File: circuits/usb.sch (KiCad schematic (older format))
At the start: 18 parts, among them J18 USB_MINI_B, Q5 Crystal_12Mhz, Q6 Q_SS8050, Q7 Q_SS8550, U10 CH340T(SSOP20W)

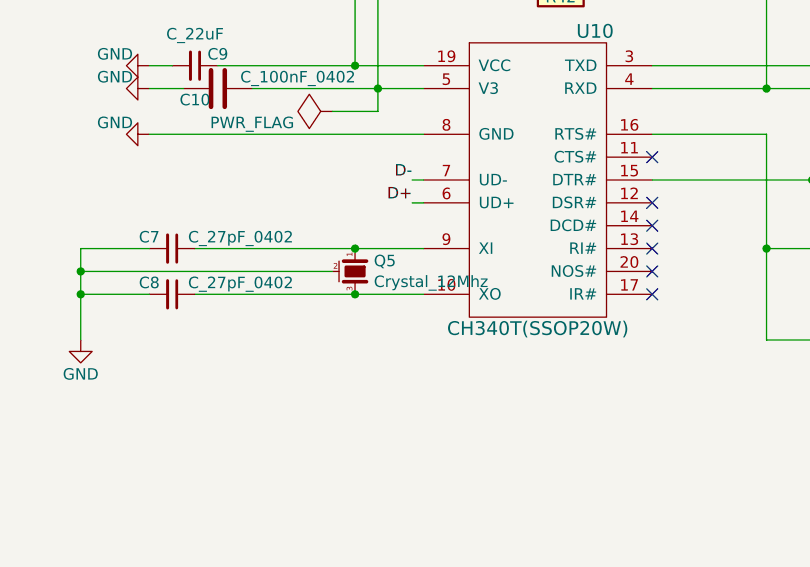
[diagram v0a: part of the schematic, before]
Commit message: finished layout, sent to board house
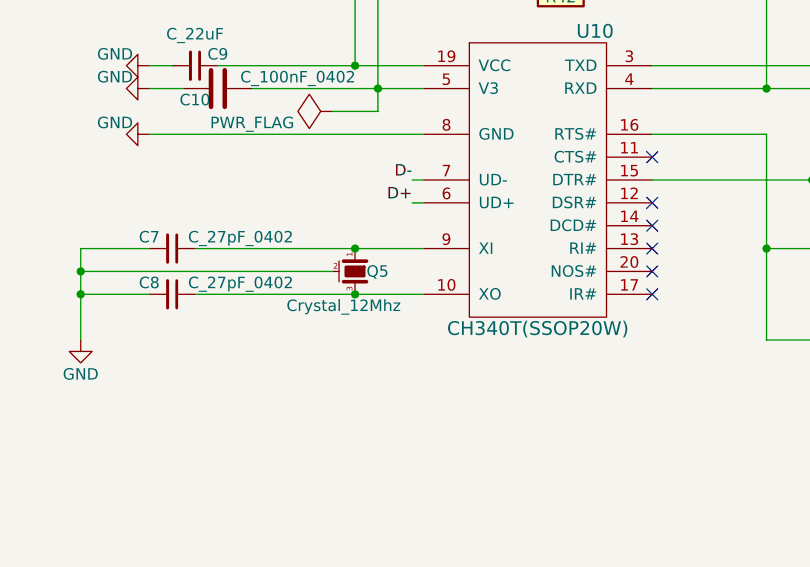
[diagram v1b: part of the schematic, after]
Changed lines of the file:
@@
 	1    0    0    -1
 $EndComp
+Wire Wire Line
+	4050 4000 4350 4000
+Wire Wire Line
+	3350 4000 4050 4000
+Connection ~ 4050 4000
+Wire Wire Line
+	4050 3800 4350 3800
+Wire Wire Line
+	3350 3800 4050 3800
+Connection ~ 4050 3800
 $Comp
 L Open_Automation:Crystal_12Mhz Q5
-U 1 1 613C96CC
+U 1 1 6045824B
 P 4050 3900
-F 0 "Q5" V 4004 3982 50  0000 L CNN
-F 1 "Crystal_12Mhz" V 4095 3982 50  0000 L CNN
-F 2 "Crystal:Crystal_SMD_3225-4Pin_3.2x2.5mm_HandSoldering" H 4050 4200 60  0001 C CNN
+F 0 "Q5" V 4050 3950 50  0000 L CNN
+F 1 "Crystal_12Mhz" V 4200 3600 50  0000 L CNN
+F 2 "Crystal:Crystal_SMD_3225-4Pin_3.2x2.5mm_HandSoldering" H 4050 3900 60  0001 C CNN
 F 3 "https://datasheet.lcsc.com/szlcsc/Yangxing-Tech-X322512MSB4SI_C9002.pdf" H 4050 3900 60  0001 C CNN
-F 4 "X322512MSB4SI" H 4050 4100 50  0001 C CNN "Part Number"
-F 5 "C9002" H 4050 4300 50  0001 C CNN "LCSC"
+F 4 "X322512MSB4SI" H 4050 3900 50  0001 C CNN "Part Number"
+F 5 "C9002" H 4050 3900 50  0001 C CNN "LCSC"
 	1    4050 3900
 	0    1    1    0
 $EndComp
-Wire Wire Line
-	3350 3800 4050 3800
-Wire Wire Line
-	3350 4000 4050 4000
-Connection ~ 4050 3800
-Wire Wire Line
-	4050 3800 4350 3800
-Connection ~ 4050 4000
-Wire Wire Line
-	4050 4000 4350 4000
 $EndSCHEMATC
